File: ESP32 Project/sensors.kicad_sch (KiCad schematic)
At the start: 0 parts

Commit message: restart
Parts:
- added U6: BME280, Package_LGA:Bosch_LGA-8_2.5x2.5mm_P0.65mm_ClockwisePinNumbering, symbol Sensor:BME280
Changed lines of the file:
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@@
 	(generator_version "10.0")
 	(paper "A4")
+	(symbol
+		(lib_id "Sensor:BME280")
+		(at 44.45 45.72 0)
+		(unit 1)
+		(body_style 1)
+		(exclude_from_sim no)
+		(in_bom yes)
+		(on_board yes)
+		(in_pos_files yes)
+		(dnp no)
+		(fields_autoplaced yes)
+		(property "Reference" "U6"
+			(at 33.02 44.4499 0)
+			(show_name no)
+			(do_not_autoplace no)
+			(effects
+				(font
+					(size 1.27 1.27)
+				)
+				(justify right)
+			)
+		)
+		(property "Value" "BME280"
+			(at 33.02 46.9899 0)
+			(show_name no)
+			(do_not_autoplace no)
+			(effects
+				(font
+					(size 1.27 1.27)
+				)
+				(justify right)
+			)
+		)
+		(property "Footprint" "Package_LGA:Bosch_LGA-8_2.5x2.5mm_P0.65mm_ClockwisePinNumbering"
+			(at 82.55 57.15 0)
+			(hide yes)
+			(show_name no)
+			(do_not_autoplace no)
+			(effects
+				(font
+					(size 1.27 1.27)
+				)
+			)
+		)
+		(property "Datasheet" "https://www.bosch-sensortec.com/media/boschsensortec/downloads/datasheets/bst-bme280-ds002.pdf"
+			(at 44.45 50.8 0)
+			(hide yes)
+			(show_name no)
+			(do_not_autoplace no)
+			(effects
+				(font
+					(size 1.27 1.27)
+				)
+			)
+		)
+		(property "Description" "3-in-1 sensor, humidity, pressure, temperature, I2C and SPI interface, 1.71-3.6V, LGA-8"
+			(at 44.45 45.72 0)
+			(hide yes)
+			(show_name no)
+			(do_not_autoplace no)
+			(effects
+				(font
+					(size 1.27 1.27)
+				)
+			)
+		)
+		(pin "7"
+		)
+		(pin "1"
+		)
+		(pin "8"
+		)
+		(pin "3"
+		)
+		(pin "4"
+		)
+		(pin "5"
+		)
+		(pin "2"
+		)
+		(pin "6"
+		)
+		(instances
+			(project "ESP32 Project"
+				(path "/52b8cc89-874f-4cef-9400-6a059fb6c311/6085c309-5041-4ae1-96f0-edf60409793b/03b1f1e9-8a18-4af6-9122-b075f5380c8d"
+					(reference "U6")
+					(unit 1)
+				)
+			)
+		)
+	)
 )

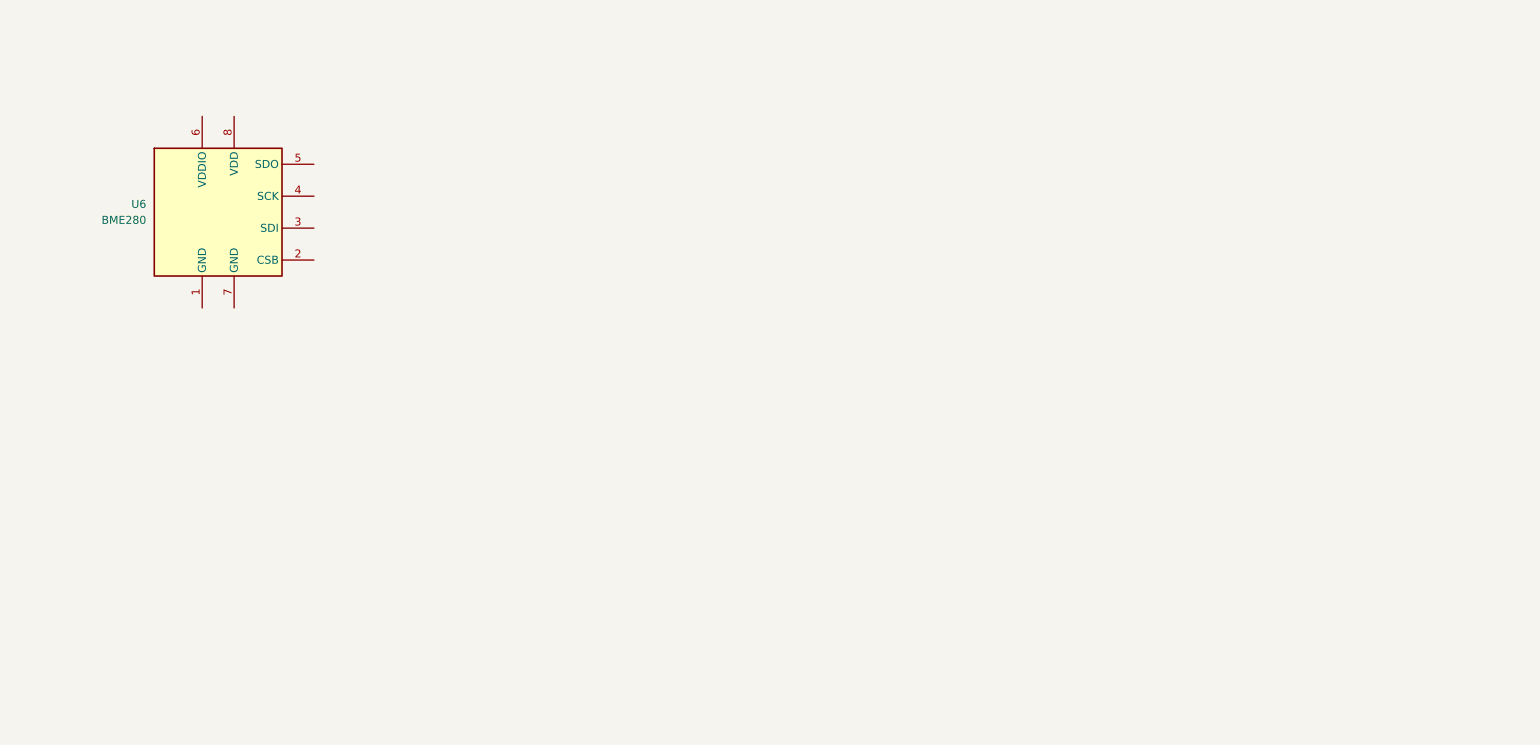
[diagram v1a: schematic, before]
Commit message: little bit of work done like bm280
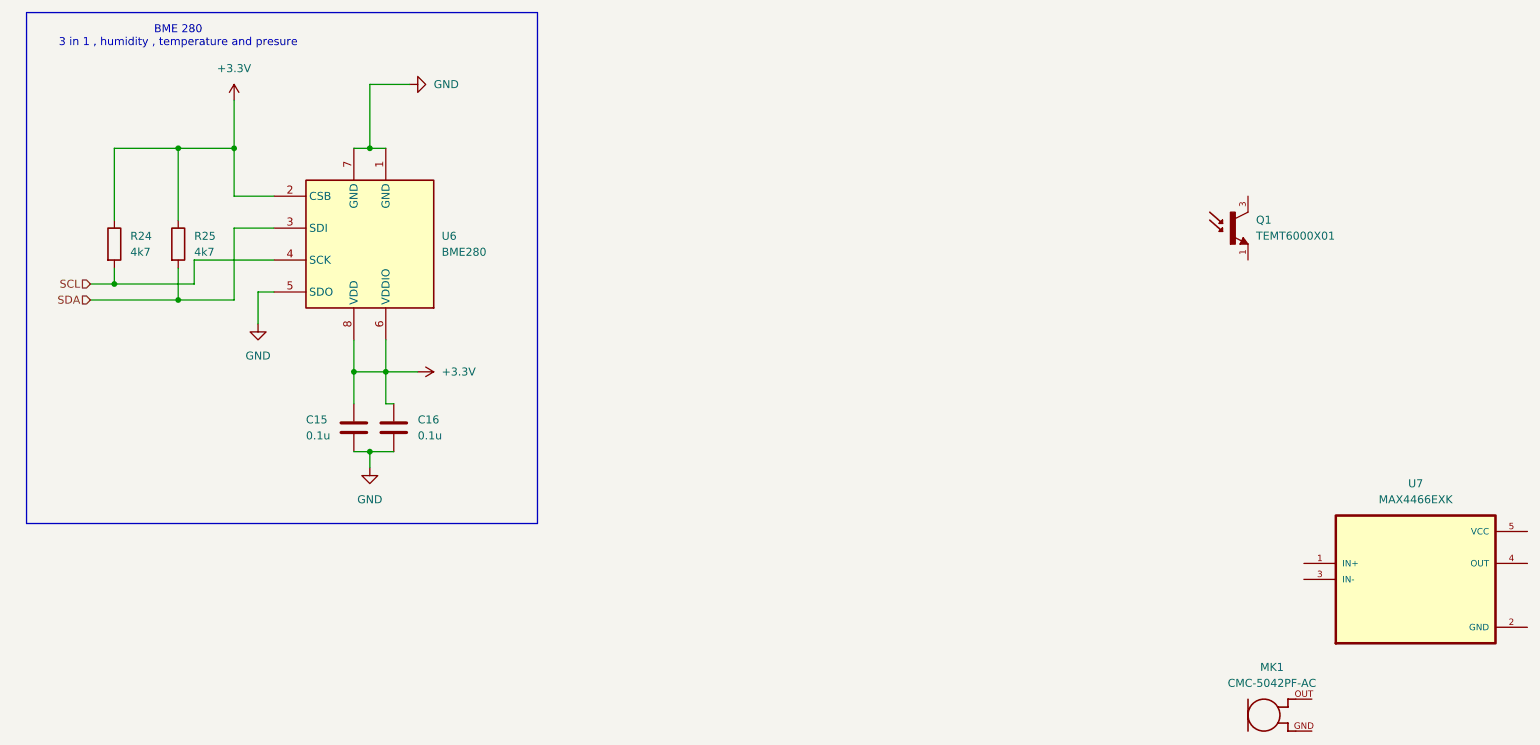
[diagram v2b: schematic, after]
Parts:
- added C15, C16: 0.1u, symbol Device:C
- added MK1: CMC-5042PF-AC, CMC-5042PF-AC:CUI_CMC-5042PF-AC, symbol CMC-5042PF-AC:CMC-5042PF-AC
- added Q1: TEMT6000X01, TEMT6000X01:TRANS_TEMT6000X01, symbol TEMT6000X01:TEMT6000X01
- added R24, R25: 4k7, symbol Device:R
- added U7: MAX4466EXK, MAX4466EXK:SOT65P210X110-5N, symbol MAX4466EXK:MAX4466EXK
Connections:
- net GND: now reaches U6.1 (GND)
- net GND: now also U6.5 (SDO), U6.7 (GND), C15.1, C16.1
- net +3.3V: now reaches U6.2 (CSB)
- net +3.3V: now also U6.6 (VDDIO), U6.8 (VDD), C15.2, C16.2, R24.1, R25.1
- net SDA: now reaches U6.3 (SDI)
- net SDA: now also R25.2
- net SCL: now reaches U6.4 (SCK)
- net SCL: now also R24.2
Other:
- note added: "BME 280 3 in 1 , humidity , temperature and presure"
- moved on the sheet: U6
